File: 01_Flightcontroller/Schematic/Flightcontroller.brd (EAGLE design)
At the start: 63.5 x 61.9 mm, 89 parts, among them IC1 FT232RL, IC2 MPU6000, IC3 BMP280, J1 2908-05WB-MG, U1 STM32F7X2RXT, U2 ATMEGA328P_TQFP, U3 LM3940IMPX-3.3/NOPB, U4 TXB0104, Y1 8MHz, Y2 16MHz

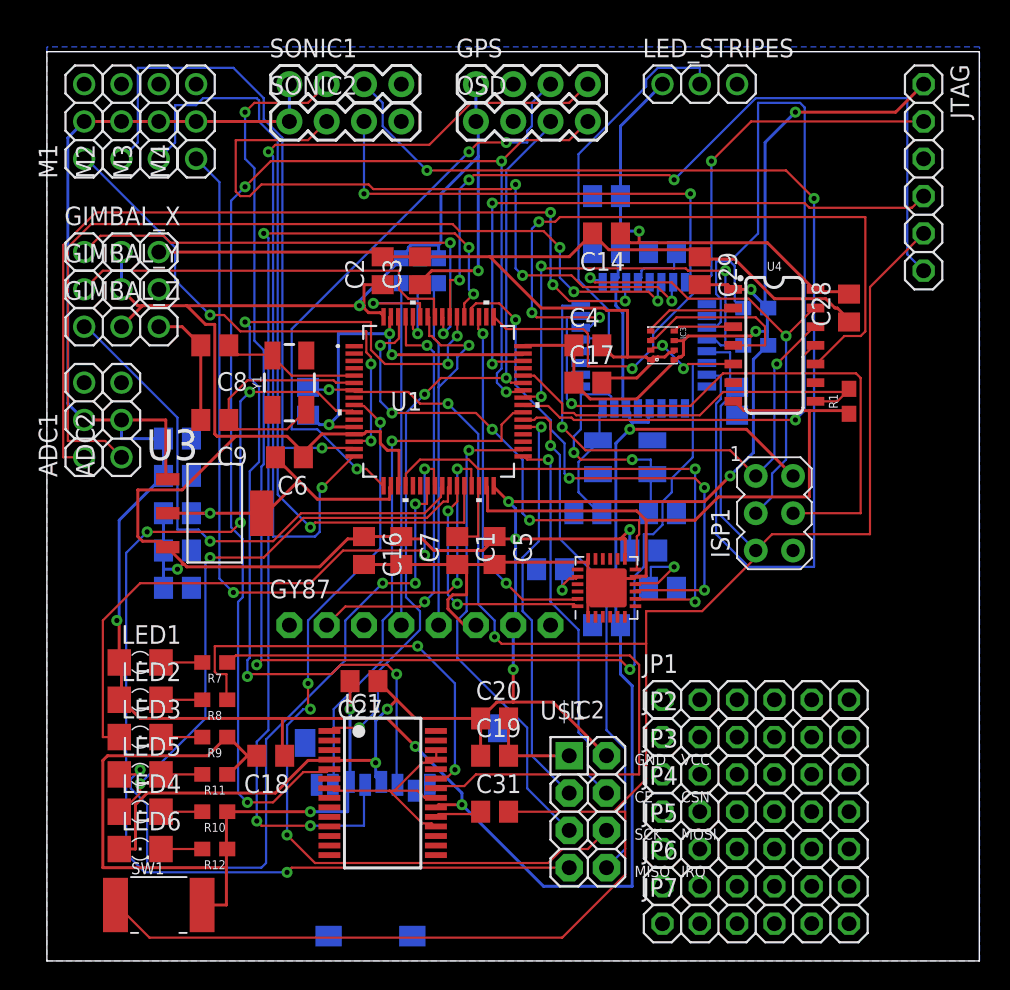
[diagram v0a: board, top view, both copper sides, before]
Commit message: Richtiges routen hilfe durch bruno
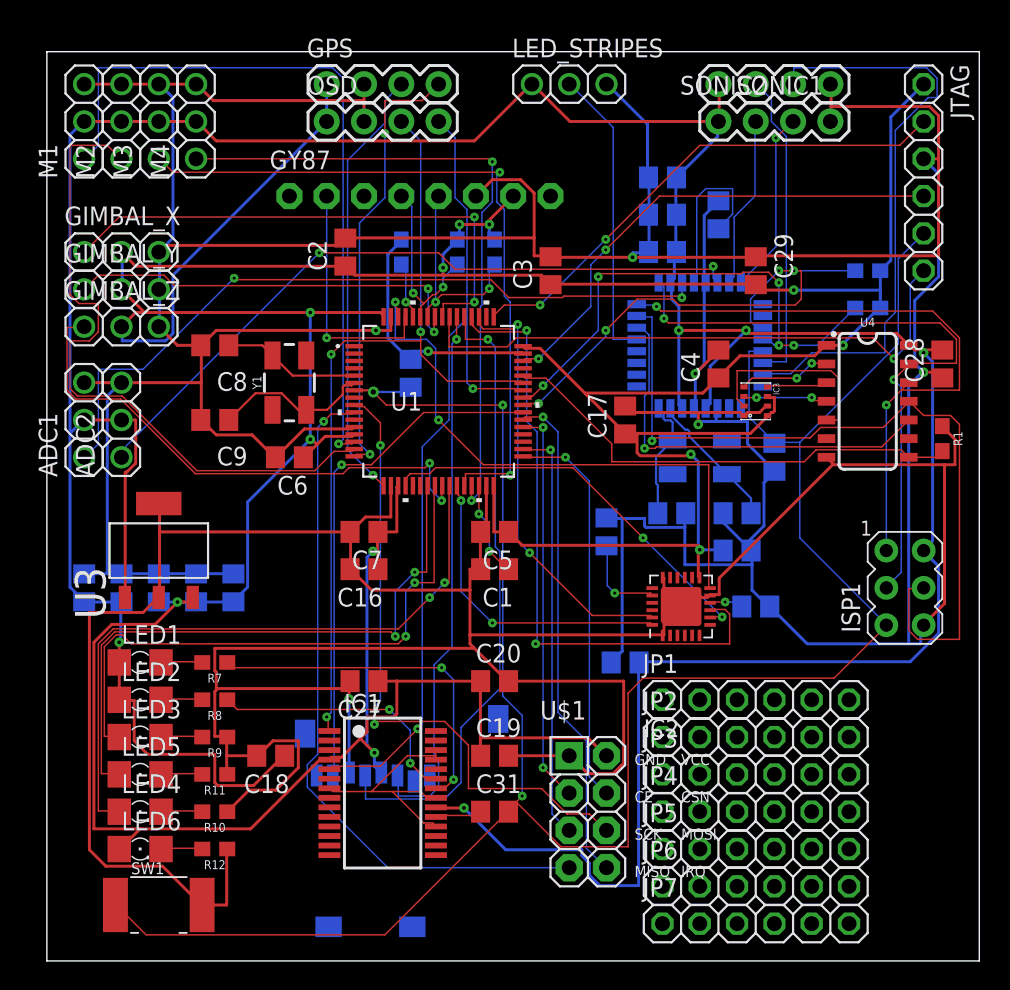
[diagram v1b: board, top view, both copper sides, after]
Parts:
- moved GY87 29.2 mm to (19.1, 91.4)
- moved SONIC1 29.2 mm to (39.4, 99.1)
- moved SONIC2 29.2 mm to (39.4, 96.5)
- moved C34 12.0 mm to (-3.81, 64.8), turned to 90 degrees
- moved ISP1 10.2 mm to (52.1, 64.8)
- moved GPS 10.2 mm to (12.7, 99.1)
- moved OSD 10.2 mm to (12.7, 96.5)
- moved C4 8.98 mm to (39.4, 80.0), turned to 90 degrees
- moved C3 8.89 mm to (27.9, 86.4)
- moved LED_STRIPES 8.89 mm to (29.2, 99.1)
- moved C23 8.52 mm to (-1.27, 64.8), turned to 90 degrees
- moved R2 8.03 mm to (49.5, 86.4)
- moved R3 8.03 mm to (49.5, 83.8)
- moved U4 7.41 mm to (49.5, 77.5)
- moved C28 7.41 mm to (54.6, 80.0)
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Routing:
- net GND: track 264.3 -> 570.1 mm, vias 6 -> 7
- net TRIGG1_IN: track 94.5 -> 21.4 mm, vias 3 -> 0
- net VCC: track 289.1 -> 332.4 mm, vias 13 -> 12
- net ECHO1_IN: track 79.3 -> 40.7 mm, vias 2 -> 0
- net VCC_2: track 207.6 -> 245.9 mm
- net TRIGG2_IN: track 48.6 -> 11.7 mm, vias 3 -> 0
- net UART1_TX: track 92.1 -> 59.1 mm, vias 4 -> 2
- net I2C2_SDA: track 65.3 -> 35.4 mm, vias 1 -> 4
- net UART2_TX: track 59.4 -> 30.3 mm
- net SPI2_MISO: track 76.8 -> 47.8 mm, vias 4 -> 1
- net SD1_CK: track 70.2 -> 43.3 mm, vias 5 -> 1
- net LED_TX: track 50.3 -> 24.1 mm, vias 0 -> 2
- net SD1_CMD: track 62.8 -> 37.2 mm, vias 5 -> 1
- net ECHO2_IN: track 33.3 -> 12.4 mm, vias 2 -> 1
- net A_SPI_NSS: track 47.2 -> 27.7 mm, vias 3 -> 1
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- removed copper zone on layer 16, net GND
